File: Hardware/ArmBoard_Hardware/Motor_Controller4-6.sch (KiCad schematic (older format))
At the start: 27 parts

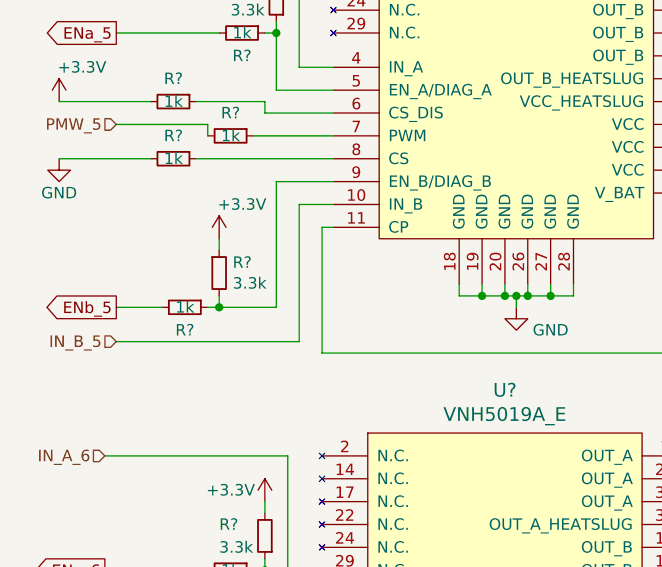
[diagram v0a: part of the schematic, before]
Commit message: ENx_# Updated
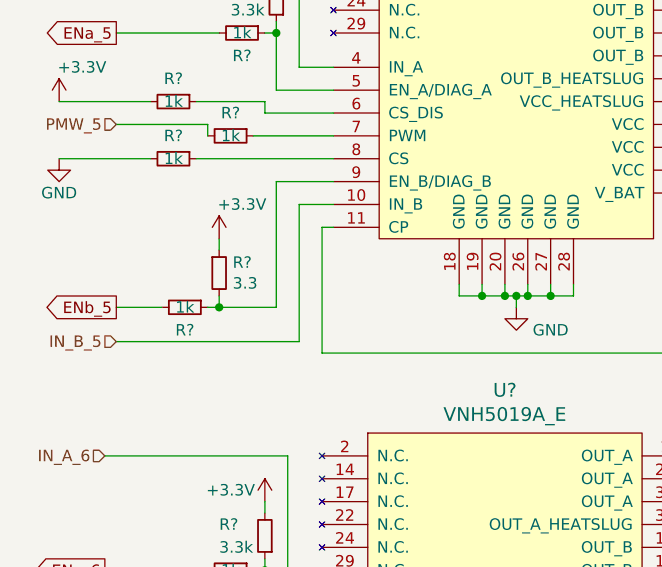
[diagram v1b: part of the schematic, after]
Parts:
- R?: value 3.3k -> 3.3
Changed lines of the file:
@@
 AR Path="/63845FEF/637AF810" Ref="R?"  Part="1"
 F 0 "R?" H 2559 4796 50  0000 L CNN
-F 1 "3.3k" H 2559 4705 50  0000 L CNN
+F 1 "3.3" H 2559 4705 50  0000 L CNN
 F 2 "" H 2500 4750 50  0001 C CNN
 F 3 "~" H 2500 4750 50  0001 C CNN
